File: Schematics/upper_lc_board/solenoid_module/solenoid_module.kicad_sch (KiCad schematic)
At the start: 16 parts

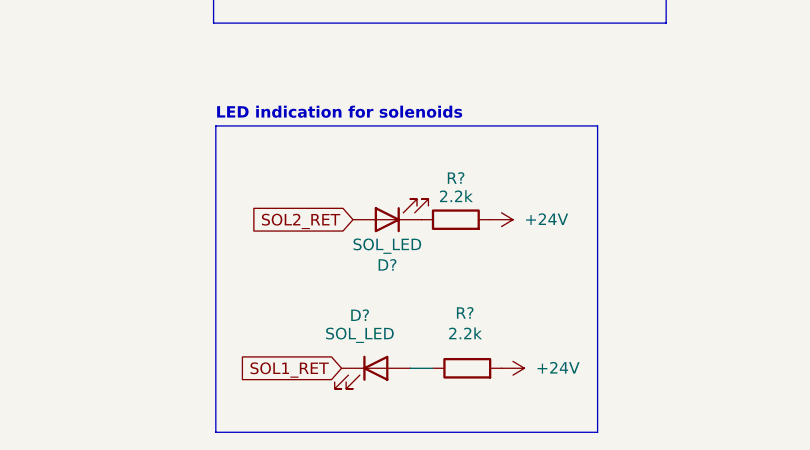
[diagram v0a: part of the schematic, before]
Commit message: reviewing schematics
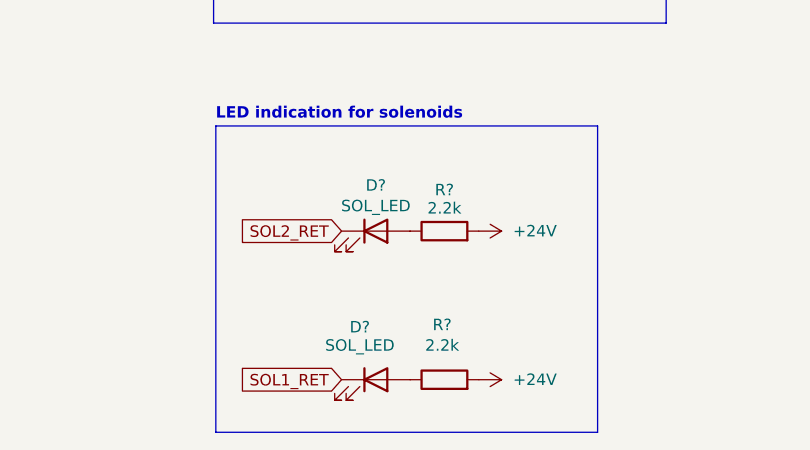
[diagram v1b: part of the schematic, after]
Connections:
- net SOL2_RET: now also D?.1 (K); no longer D?.2 (A)
- net at R?.1: now also D?.2 (A); no longer D?.1 (K)
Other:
- moved on the sheet: D?, R?
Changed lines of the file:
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@@
-	(wire
-		(pts
-			(xy 101.6 140.97) (xy 99.06 140.97)
-		)
-		(stroke
-			(width 0)
-			(type default)
-		)
-	)
 	(wire
 		(pts
@@
 	(global_label "SOL1_RET"
 		(shape input)
-		(at 91.44 140.97 180)
+		(at 91.44 142.24 180)
 		(fields_autoplaced yes)
 		(effects
@@
 		)
 		(property "Intersheetrefs" "${INTERSHEET_REFS}"
-			(at 79.323 140.97 0)
+			(at 79.323 142.24 0)
 			(effects
 				(font
@@
 	(global_label "SOL2_RET"
 		(shape input)
-		(at 92.71 124.46 180)
+		(at 91.44 125.73 180)
 		(fields_autoplaced yes)
 		(effects
@@
 		)
 		(property "Intersheetrefs" "${INTERSHEET_REFS}"
-			(at 80.593 124.46 0)
+			(at 79.323 125.73 0)
 			(effects
 				(font
@@
 	(symbol
 		(lib_id "Device:LED")
-		(at 96.52 124.46 180)
+		(at 95.25 125.73 0)
 		(unit 1)
 		(exclude_from_sim no)
@@
 		(dnp no)
 		(property "Reference" "D?"
-			(at 96.52 129.54 0)
+			(at 95.25 120.65 0)
 			(effects
 				(font
@@
 		)
 		(property "Value" "SOL_LED"
-			(at 96.52 127.254 0)
+			(at 95.25 122.936 0)
 			(effects
 				(font
@@
 		)
 		(property "Footprint" "LED_SMD:LED_0805_2012Metric"
-			(at 96.52 124.46 0)
+			(at 95.25 125.73 0)
 			(effects
 				(font
@@
 		)
 		(property "Datasheet" "~"
-			(at 96.52 124.46 0)
+			(at 95.25 125.73 0)
 			(effects
 				(font
@@
 		)
 		(property "Description" "Light emitting diode"
-			(at 96.52 124.46 0)
+			(at 95.25 125.73 0)
 			(effects
 				(font
@@
 	(symbol
 		(lib_id "power:+24V")
-		(at 107.95 124.46 270)
+		(at 106.68 125.73 270)
 		(unit 1)
 		(exclude_from_sim no)
@@
 		(fields_autoplaced yes)
 		(property "Reference" "#PWR?"
-			(at 104.14 124.46 0)
+			(at 102.87 125.73 0)
 			(effects
 				(font
@@
 		)
 		(property "Value" "+24V"
-			(at 111.76 124.4601 90)
+			(at 110.49 125.7301 90)
 			(effects
 				(font
@@
 		)
 		(property "Footprint" ""
-			(at 107.95 124.46 0)
+			(at 106.68 125.73 0)
 			(effects
 				(font
@@
 		)
 		(property "Datasheet" ""
-			(at 107.95 124.46 0)
+			(at 106.68 125.73 0)
 			(effects
 				(font
@@
 		)
 		(property "Description" "Power symbol creates a global label with name \"+24V\""
-			(at 107.95 124.46 0)
+			(at 106.68 125.73 0)
 			(effects
 				(font
@@
 	(symbol
 		(lib_id "Device:R")
-		(at 105.41 140.97 90)
+		(at 102.87 142.24 90)
 		(unit 1)
 		(exclude_from_sim no)
@@
 		(dnp no)
 		(property "Reference" "R?"
-			(at 105.156 134.874 90)
+			(at 102.616 136.144 90)
 			(effects
 				(font
@@
 		)
 		(property "Value" "2.2k"
-			(at 105.156 137.16 90)
+			(at 102.616 138.43 90)
 			(effects
 				(font
@@
 		)
 		(property "Footprint" "Resistor_SMD:R_1210_3225Metric"
-			(at 105.41 142.748 90)
+			(at 102.87 144.018 90)
 			(effects
 				(font
@@
 		)
 		(property "Datasheet" "~"
-			(at 105.41 140.97 0)
+			(at 102.87 142.24 0)
 			(effects
 				(font
@@
 		)
 		(property "Description" "Current Limiting Resistor"
-			(at 105.41 140.97 0)
+			(at 102.87 142.24 0)
 			(effects
 				(font
@@
 	(symbol
 		(lib_id "power:+24V")
-		(at 109.22 140.97 270)
+		(at 106.68 142.24 270)
 		(unit 1)
 		(exclude_from_sim no)
@@
 		(fields_autoplaced yes)
 		(property "Reference" "#PWR?"
-			(at 105.41 140.97 0)
+			(at 102.87 142.24 0)
 			(effects
 				(font
@@
 		)
 		(property "Value" "+24V"
-			(at 113.03 140.9701 90)
+			(at 110.49 142.2401 90)
 			(effects
 				(font
@@
 		)
 		(property "Footprint" ""
-			(at 109.22 140.97 0)
+			(at 106.68 142.24 0)
 			(effects
 				(font
@@
 		)
 		(property "Datasheet" ""
-			(at 109.22 140.97 0)
+			(at 106.68 142.24 0)
 			(effects
 				(font
@@
 		)
 		(property "Description" "Power symbol creates a global label with name \"+24V\""
-			(at 109.22 140.97 0)
+			(at 106.68 142.24 0)
 			(effects
 				(font
@@
 	(symbol
 		(lib_id "Device:R")
-		(at 104.14 124.46 90)
+		(at 102.87 125.73 90)
 		(unit 1)
 		(exclude_from_sim no)
@@
 		(dnp no)
 		(property "Reference" "R?"
-			(at 104.14 119.888 90)
+			(at 102.87 121.158 90)
 			(effects
 				(font
@@
 		)
 		(property "Value" "2.2k"
-			(at 104.14 121.92 90)
+			(at 102.87 123.19 90)
 			(effects
 				(font
@@
 		)
 		(property "Footprint" "Resistor_SMD:R_1210_3225Metric"
-			(at 104.14 126.238 90)
+			(at 102.87 127.508 90)
 			(effects
 				(font
@@
 		)
 		(property "Datasheet" "~"
-			(at 104.14 124.46 0)
+			(at 102.87 125.73 0)
 			(effects
 				(font
@@
 		)
 		(property "Description" "Current Limiting Resistor"
-			(at 104.14 124.46 0)
+			(at 102.87 125.73 0)
 			(effects
 				(font
@@
 	(symbol
 		(lib_id "Device:LED")
-		(at 95.25 140.97 0)
+		(at 95.25 142.24 0)
 		(unit 1)
 		(exclude_from_sim no)
@@
 		(dnp no)
 		(property "Reference" "D?"
-			(at 93.472 135.128 0)
+			(at 93.472 136.398 0)
 			(effects
 				(font
@@
 		)
 		(property "Value" "SOL_LED"
-			(at 93.472 137.16 0)
+			(at 93.472 138.43 0)
 			(effects
 				(font
@@
 		)
 		(property "Footprint" "LED_SMD:LED_0805_2012Metric"
-			(at 95.25 140.97 0)
+			(at 95.25 142.24 0)
 			(effects
 				(font
@@
 		)
 		(property "Datasheet" "~"
-			(at 95.25 140.97 0)
+			(at 95.25 142.24 0)
 			(effects
 				(font
@@
 		)
 		(property "Description" "Light emitting diode"
-			(at 95.25 140.97 0)
-			(effects
-				(font
+			(at 95.25 142.24 0)
+			(effects
+				(font

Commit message: temp commit for layout work
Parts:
- F1: footprint (none) -> 0679L0250-05:FUSC6125X279N
- R? (x3): footprint Capacitor_SMD:C_0402_1005Metric -> Resistor_SMD:R_0402_1005Metric
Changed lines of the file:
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@@
 			)
 		)
-		(property "Footprint" "Capacitor_SMD:C_0402_1005Metric"
+		(property "Footprint" "Resistor_SMD:R_0402_1005Metric"
 			(at 168.91 88.392 90)
 			(effects
@@
 			)
 		)
-		(property "Footprint" "Capacitor_SMD:C_0402_1005Metric"
+		(property "Footprint" "Resistor_SMD:R_0402_1005Metric"
 			(at 182.118 137.16 90)
 			(effects
@@
 			)
 		)
-		(property "Footprint" "Capacitor_SMD:C_0402_1005Metric"
+		(property "Footprint" "Resistor_SMD:R_0402_1005Metric"
 			(at 168.91 131.572 90)
 			(effects
@@
 			)
 		)
-		(property "Footprint" ""
+		(property "Footprint" "0679L0250-05:FUSC6125X279N"
 			(at 98.552 49.53 90)
 			(effects
